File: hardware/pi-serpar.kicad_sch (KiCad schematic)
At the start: 31 parts, among them J2 40HAT, J3 IEEE1284, J4 IEEE1284, J5 RS232, J7 RS232, U1 CAT24C32, U2 SN74LVC161284DLR, U3 MAX3232

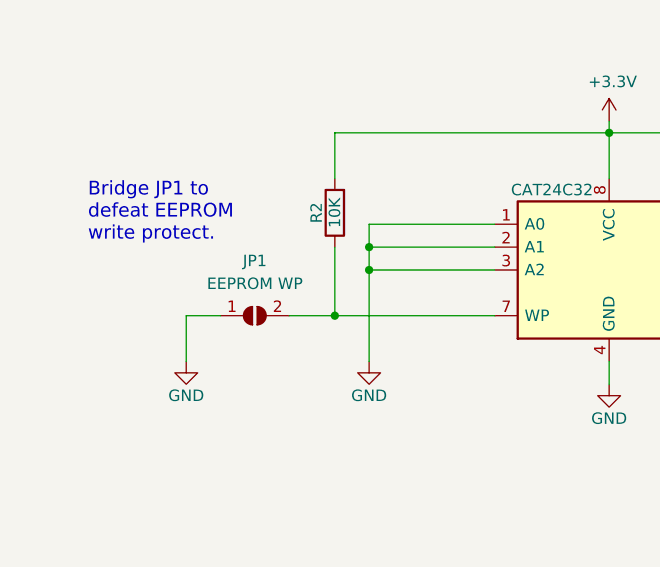
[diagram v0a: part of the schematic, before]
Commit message: v1 ordered at jlcpcb
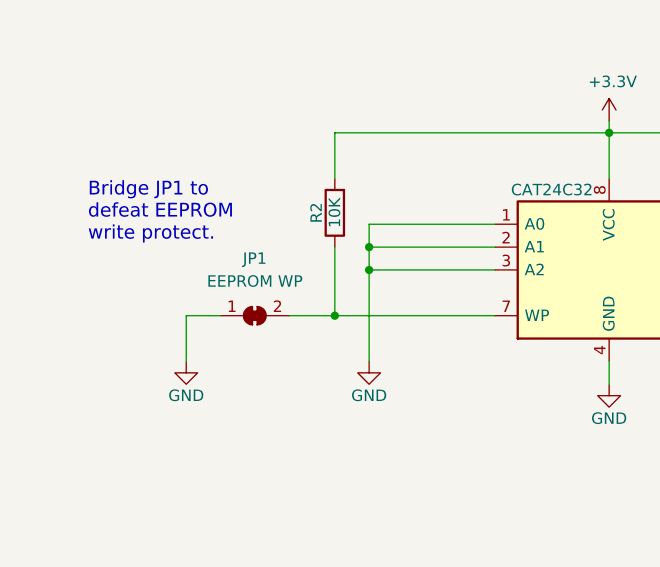
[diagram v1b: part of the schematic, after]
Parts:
- JP1: footprint Jumper:SolderJumper-2_P1.3mm_Open_RoundedPad1.0x1.5mm -> Jumper:SolderJumper-2_P1.3mm_Bridged_Pad1.0x1.5mm; symbol Jumper:SolderJumper_2_Open -> Jumper:SolderJumper_2_Bridged
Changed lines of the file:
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@@
     )
   )
-  (symbol (lib_id "Jumper:SolderJumper_2_Open") (at 40.64 190.5 0) (unit 1)
+  (symbol (lib_id "Jumper:SolderJumper_2_Bridged") (at 40.64 190.5 0) (unit 1)
     (in_bom yes) (on_board yes) (dnp no) (fields_autoplaced)
-    (property "Reference" "JP1" (at 40.64 184.404 0)
+    (property "Reference" "JP1" (at 40.64 184.15 0)
       (effects (font (size 1.27 1.27)))
     )
-    (property "Value" "EEPROM WP" (at 40.64 186.944 0)
+    (property "Value" "EEPROM WP" (at 40.64 186.69 0)
       (effects (font (size 1.27 1.27)))
     )
-    (property "Footprint" "Jumper:SolderJumper-2_P1.3mm_Open_RoundedPad1.0x1.5mm" (at 40.64 190.5 0)
+    (property "Footprint" "Jumper:SolderJumper-2_P1.3mm_Bridged_Pad1.0x1.5mm" (at 40.64 190.5 0)
       (effects (font (size 1.27 1.27)) hide)
     )
